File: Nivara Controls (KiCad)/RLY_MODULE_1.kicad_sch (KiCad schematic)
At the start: 3 parts, among them K1 DS1E-S-DC3V, K2 DS1E-S-DC3V, U1 LK1802

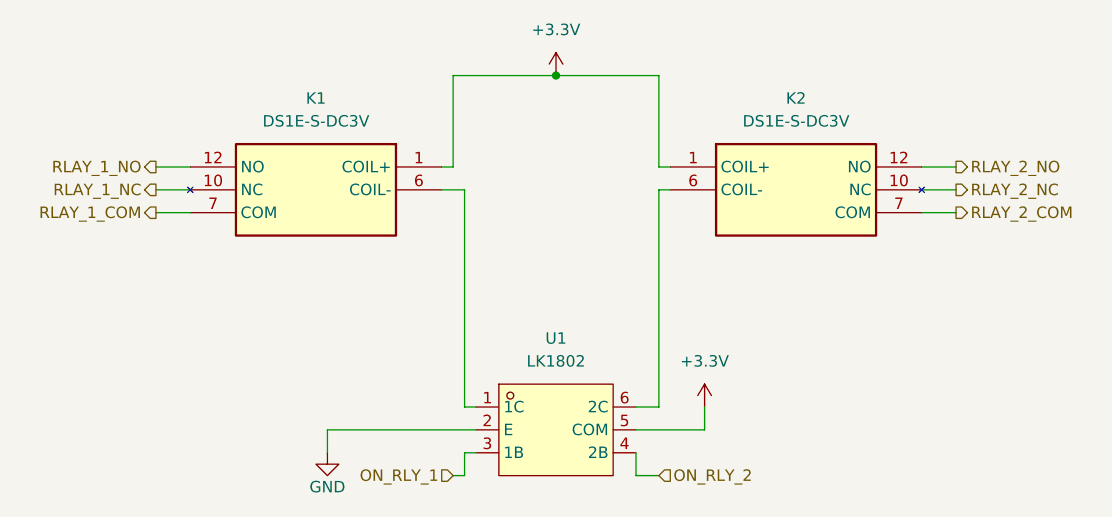
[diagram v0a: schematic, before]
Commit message: Actualization
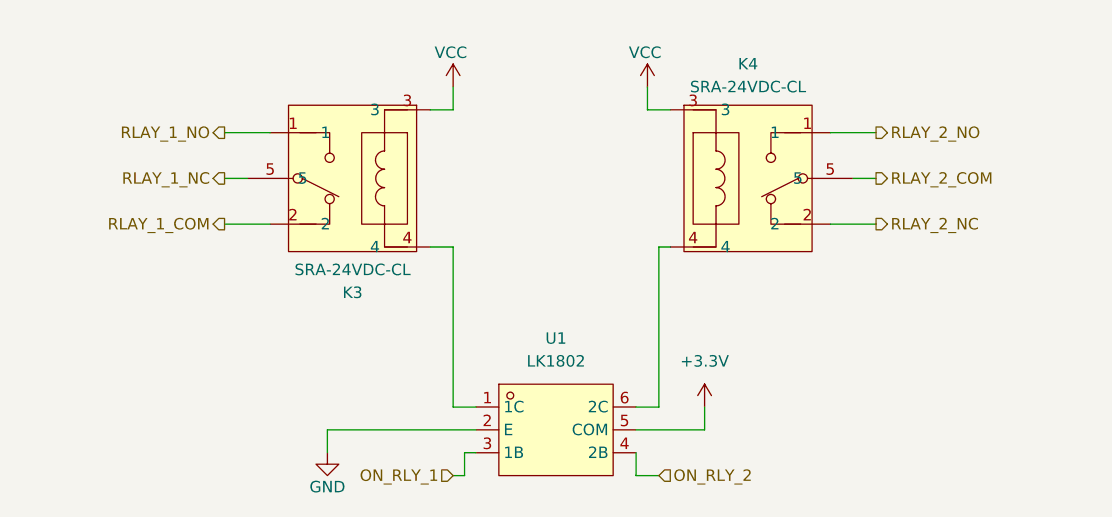
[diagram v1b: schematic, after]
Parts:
- removed K1, K2: DS1E-S-DC3V, footprints:RELAY_DS1E_PAN, symbol DS1E-S-DC3V:DS1E-S-DC3V
- added K3, K4: SRA-24VDC-CL, EastEDA:RELAY-TH_SRA-X-CX, symbol EDA:SRA-24VDC-CL
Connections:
- net RLAY_1_COM: now also K3.2
- net RLAY_1_NC: now also K3.5
- net RLAY_1_NO: now also K3.1
- net RLAY_2_COM: now also K4.5
- net RLAY_2_NC: now also K4.2
- net RLAY_2_NO: now also K4.1
- net at U1.1 (1C): now also K3.4
- net at U1.6 (2C): now also K4.4
- new net VCC: K3.3, K4.3
